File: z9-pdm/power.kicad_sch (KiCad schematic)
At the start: 12 parts, among them Q4 DMT6007LFG, U8 LM74700, U9 VN9016AJTR

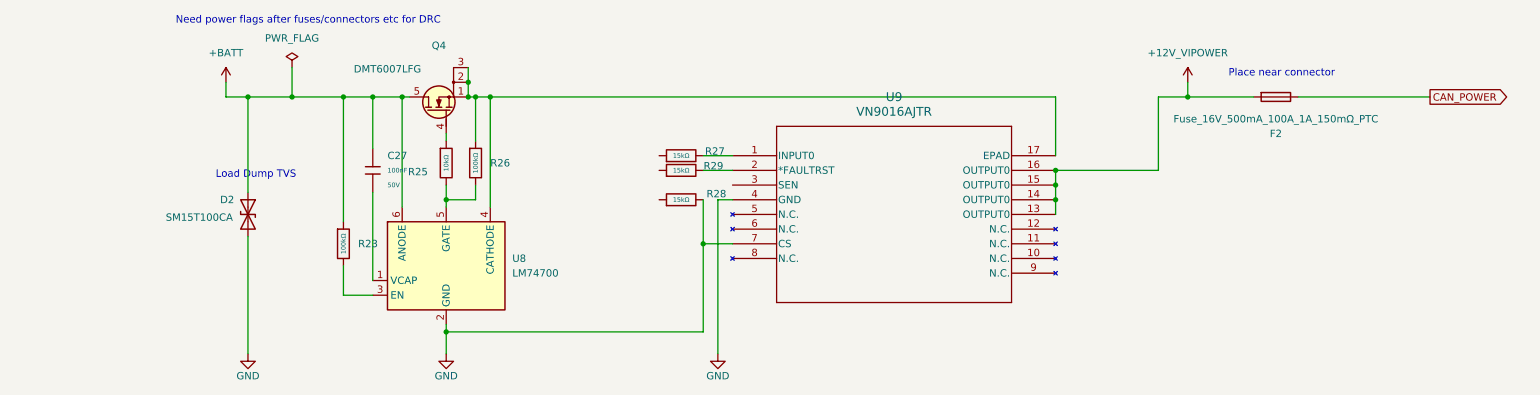
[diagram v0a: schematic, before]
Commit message: pre final pdm erc
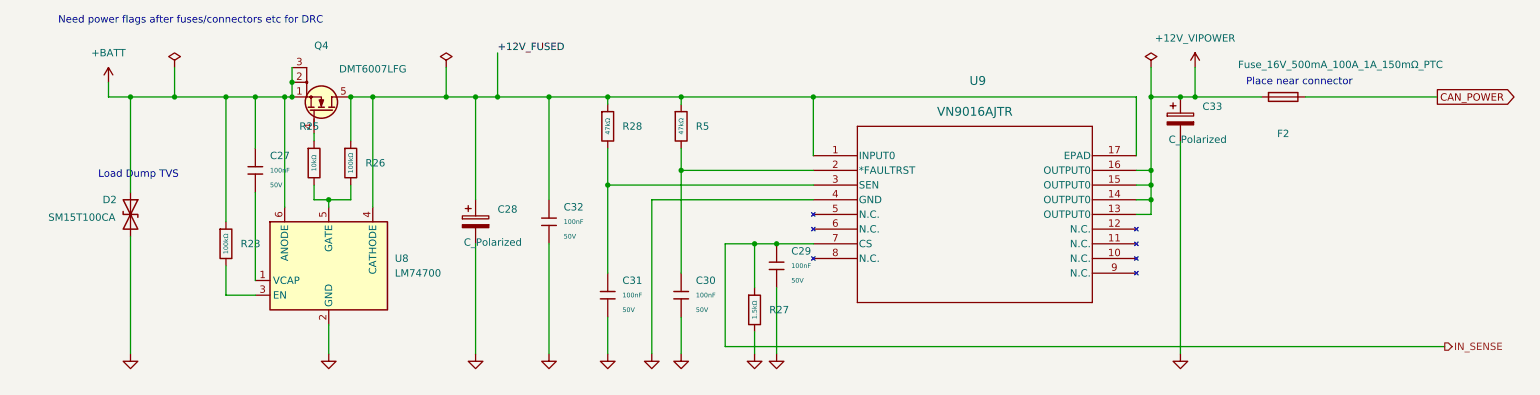
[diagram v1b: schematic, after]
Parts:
- removed R27, R28, R29: 15kΩ, PCM_JLCPCB:R_0402, symbol dnt_global:0402,15kΩ
- added C28, C33: C_Polarized, Capacitor_SMD:CP_Elec_10x10, symbol Device:C_Polarized
- added C29, C30, C31, C32: 100nF, dnt:C_0603_1608Metric, symbol dnt_global:0603 100nF 50V X7R
- added R27: 1.5kΩ, PCM_JLCPCB:R_0402, symbol PCM_JLCPCB-Resistors:0402,1.5kΩ
- added R28, R5: 47kΩ, PCM_JLCPCB:R_0603, symbol PCM_JLCPCB-Resistors:0603,47kΩ
- U9: footprint POWERSSO16_3p9X4p9X0p5_STM -> dnt:POWERSSO16_3p9X4p9X0p5_STM; LCSC C19191773 -> (none)
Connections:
- net +12V_VIPOWER: now also C33.1
- net +BATT: now also Q4.1 (S), Q4.2 (S), Q4.3 (S); no longer Q4.5 (D)
- net GND: now also C28.2, C29.2, C30.2, C31.2, C32.2, C33.2, R27.2; no longer U9.7 (CS)
- net +12V_FUSED: now reaches U9.1 (INPUT0)
- net +12V_FUSED: now also Q4.5 (D), R26.1, U8.4 (CATHODE), U9.17 (EPAD), C28.1, C32.1, R28.1, R5.1
- net at U9.2 (*FAULTRST): now also C30.1, R5.2
- net at U9.3 (SEN): now also C31.1, R28.2
- new net IN_SENSE: C29.1, R27.1, U9.7 (CS)
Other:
- moved on the sheet: C27, D2, F2, Q4, R23, R25, R26, U8, U9
